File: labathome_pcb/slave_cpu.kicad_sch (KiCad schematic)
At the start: 49 parts, among them J1 HALL, J25 TC-2030, J27 ADDA, J28 Brushless, J34 STM32 EXT, J36 PROG_STM, U16 LM358, U3 DRV8313, U5 STM32G431R8Tx

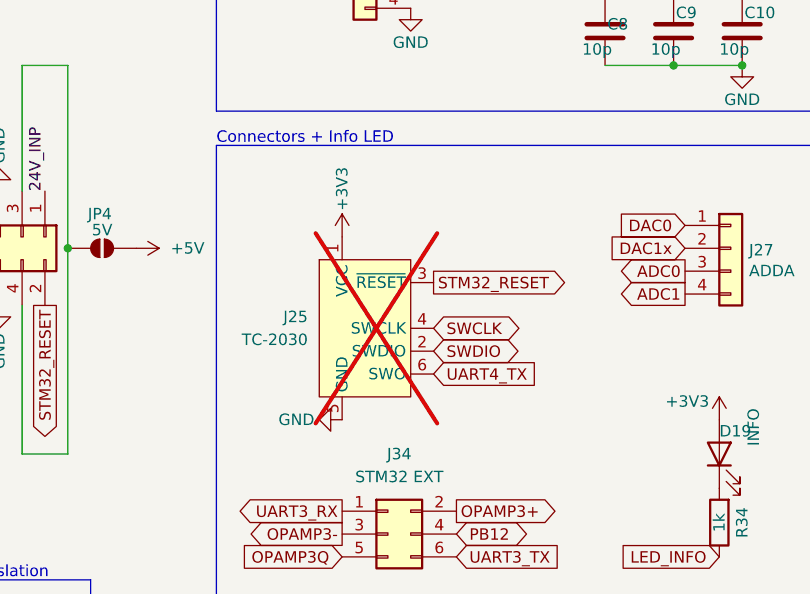
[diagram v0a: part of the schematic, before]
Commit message: Optimized PCB
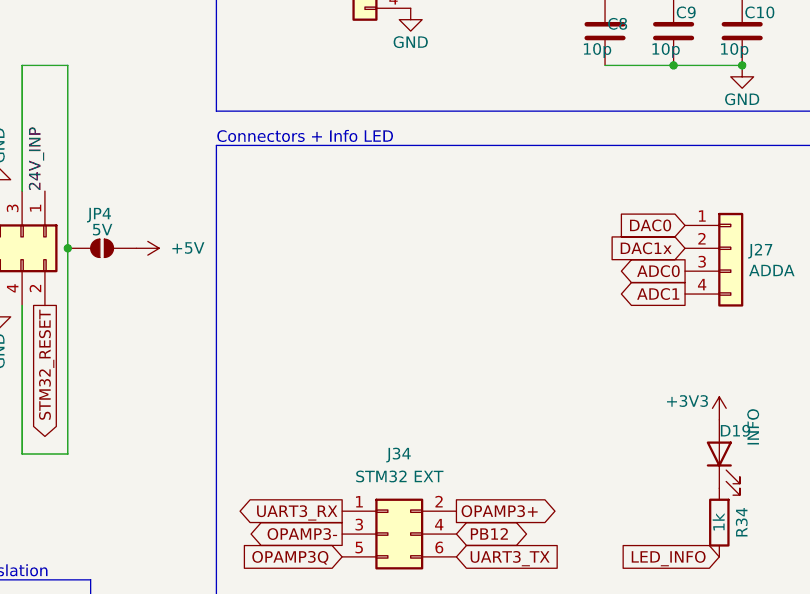
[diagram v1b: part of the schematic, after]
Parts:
- removed J25: TC-2030, Connector:Tag-Connect_TC2030-IDC-NL_2x03_P1.27mm_Vertical, symbol Connector:Conn_ARM_SWD_TagConnect_TC2030-NL
